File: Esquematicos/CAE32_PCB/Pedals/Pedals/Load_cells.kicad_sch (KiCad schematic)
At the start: 55 parts, among them J18 LC_2, J19 LC_1, J20 LC_3, Q1 MMBT3906, Q2 MMBT3906, Q3 MMBT3906, U5 HX711, U6 HX711, U7 HX711

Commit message: add: plantilla para diseño de pcb para shifter
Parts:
- Q1, Q2, Q3: Vendor (none) -> C2891809
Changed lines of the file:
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@@
+      (effects (font (size 1.27 1.27)) hide)
+    )
+    (property "Vendor" "C2891809" (id 5) (at 75.565 28.575 0)
       (effects (font (size 1.27 1.27)) hide)
     )
@@
       (effects (font (size 1.27 1.27)) hide)
     )
+    (property "Vendor" "C2891809" (id 5) (at 212.09 81.28 0)
+      (effects (font (size 1.27 1.27)) hide)
+    )
     (pin "1")
     (pin "2")
@@
       (effects (font (size 1.27 1.27)) hide)
     )
+    (property "Vendor" "C2891809" (id 5) (at 73.66 116.84 0)
+      (effects (font (size 1.27 1.27)) hide)
+    )

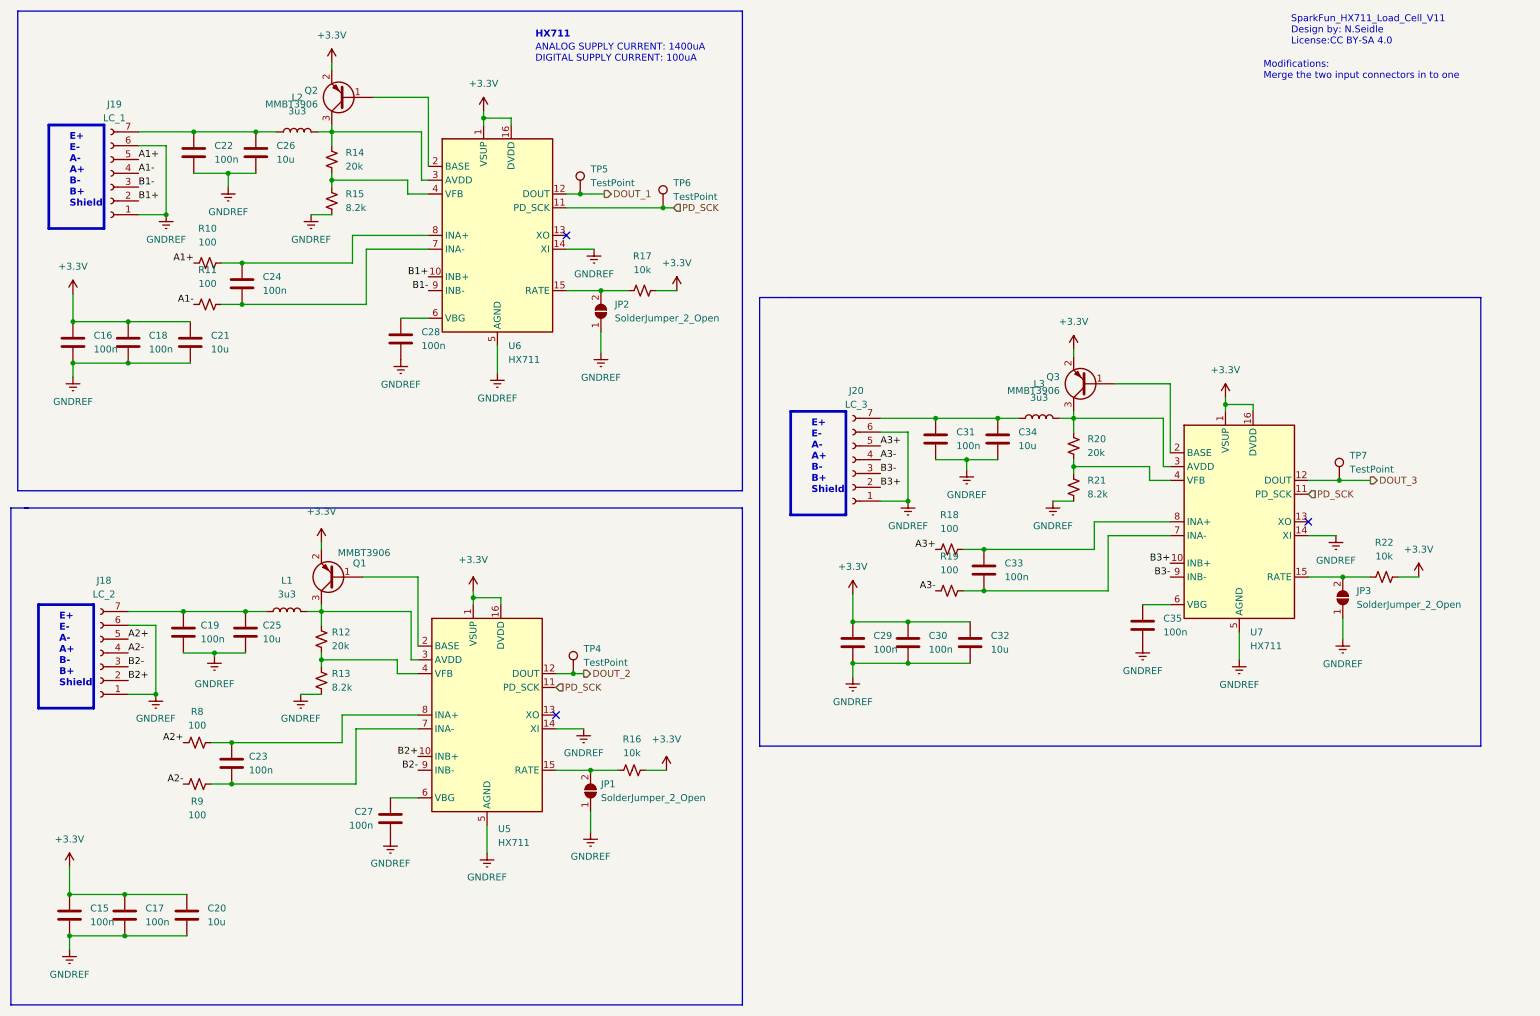
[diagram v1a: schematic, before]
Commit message: chore: arrange schematics components
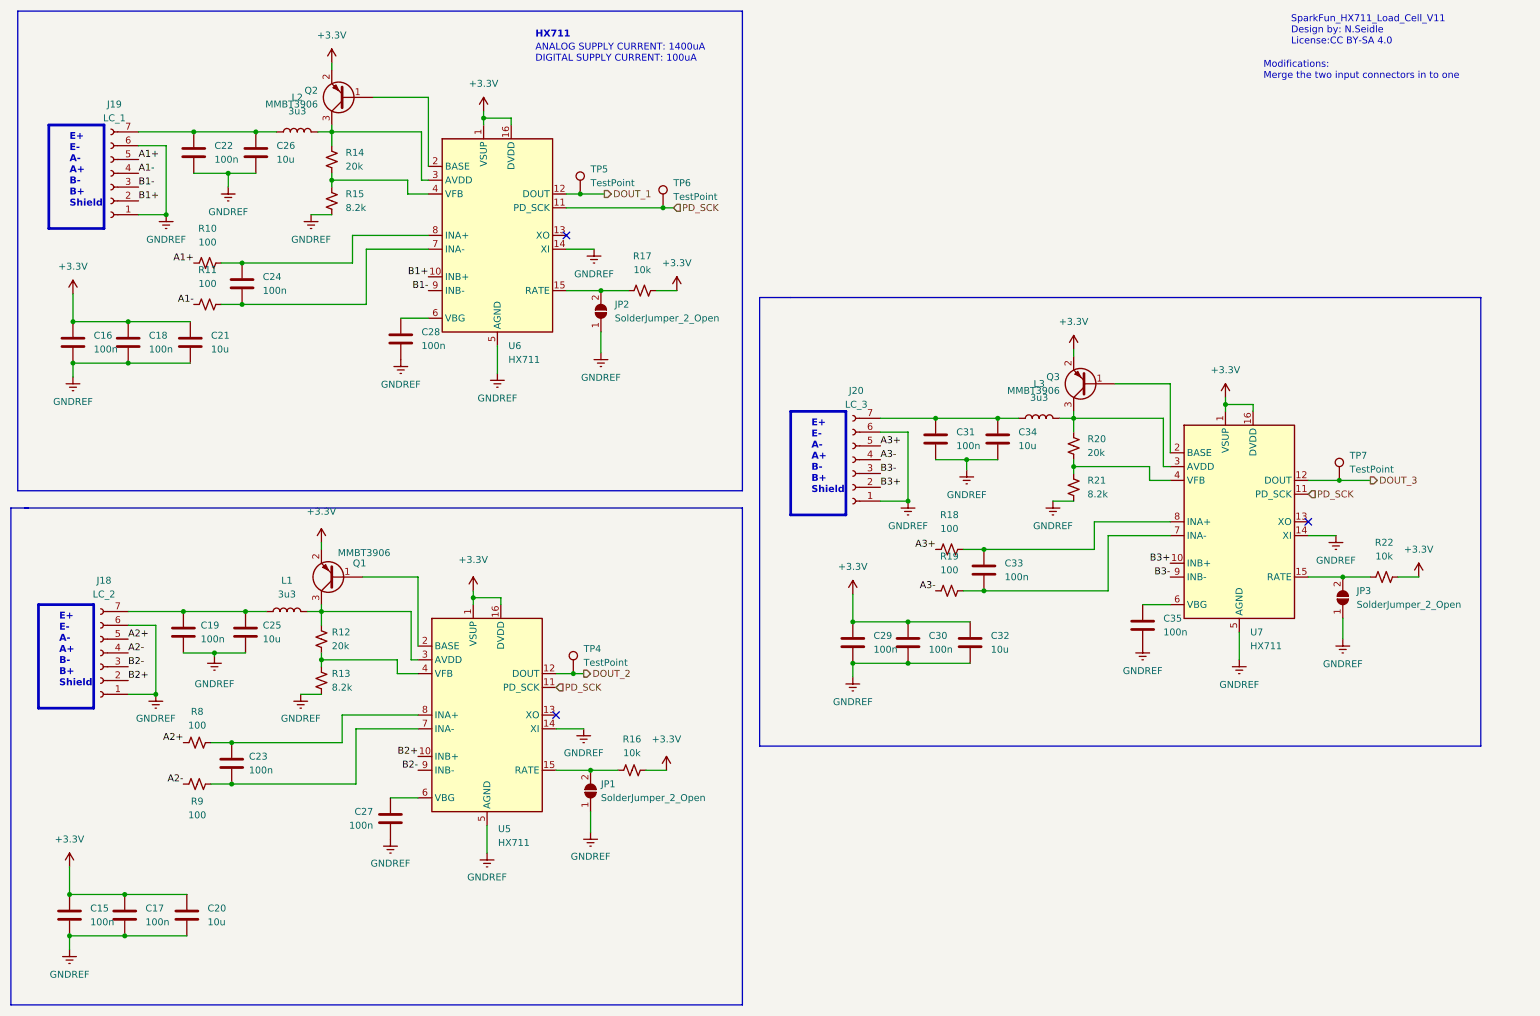
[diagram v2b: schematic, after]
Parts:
- C15, C16, C17, C18, C19, C20, C21, C22, C23, C24, C25, C26, C27, C28, C29, C30, C31, C32, C33, C34, C35: footprint Capacitor_SMD:C_0603_1608Metric_Pad1.08x0.95mm_HandSolder -> Capacitor_SMD:C_0603_1608Metric
- L1, L2, L3: footprint Inductor_SMD:L_0402_1005Metric_Pad0.77x0.64mm_HandSolder -> Inductor_SMD:L_0402_1005Metric
- R10, R11, R12, R13, R14, R15, R16, R17, R18, R19, R20, R21, R22, R8, R9: footprint Resistor_SMD:R_0603_1608Metric_Pad0.98x0.95mm_HandSolder -> Resistor_SMD:R_0603_1608Metric
